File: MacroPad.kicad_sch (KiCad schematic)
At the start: 29 parts, among them SW1 RotaryEncoder_Switch, SW12 RotaryEncoder_Switch, SW2 RotaryEncoder_Switch, U1 Pico

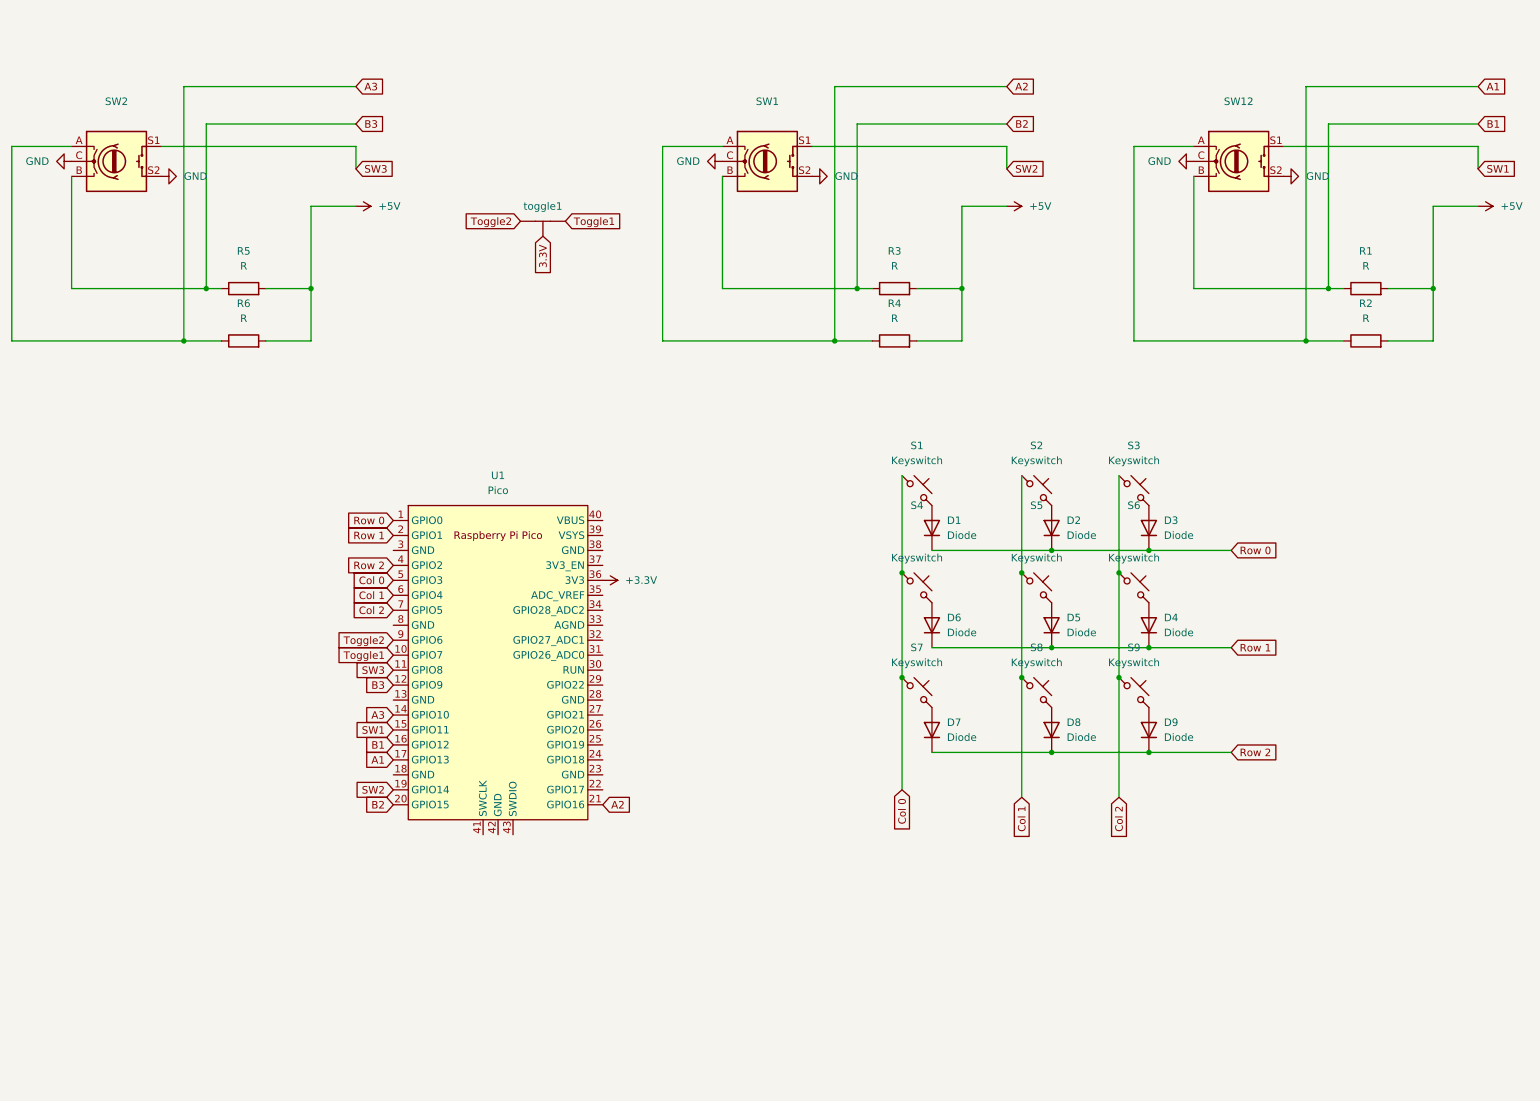
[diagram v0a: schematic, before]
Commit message: Redid the schematic should be finished
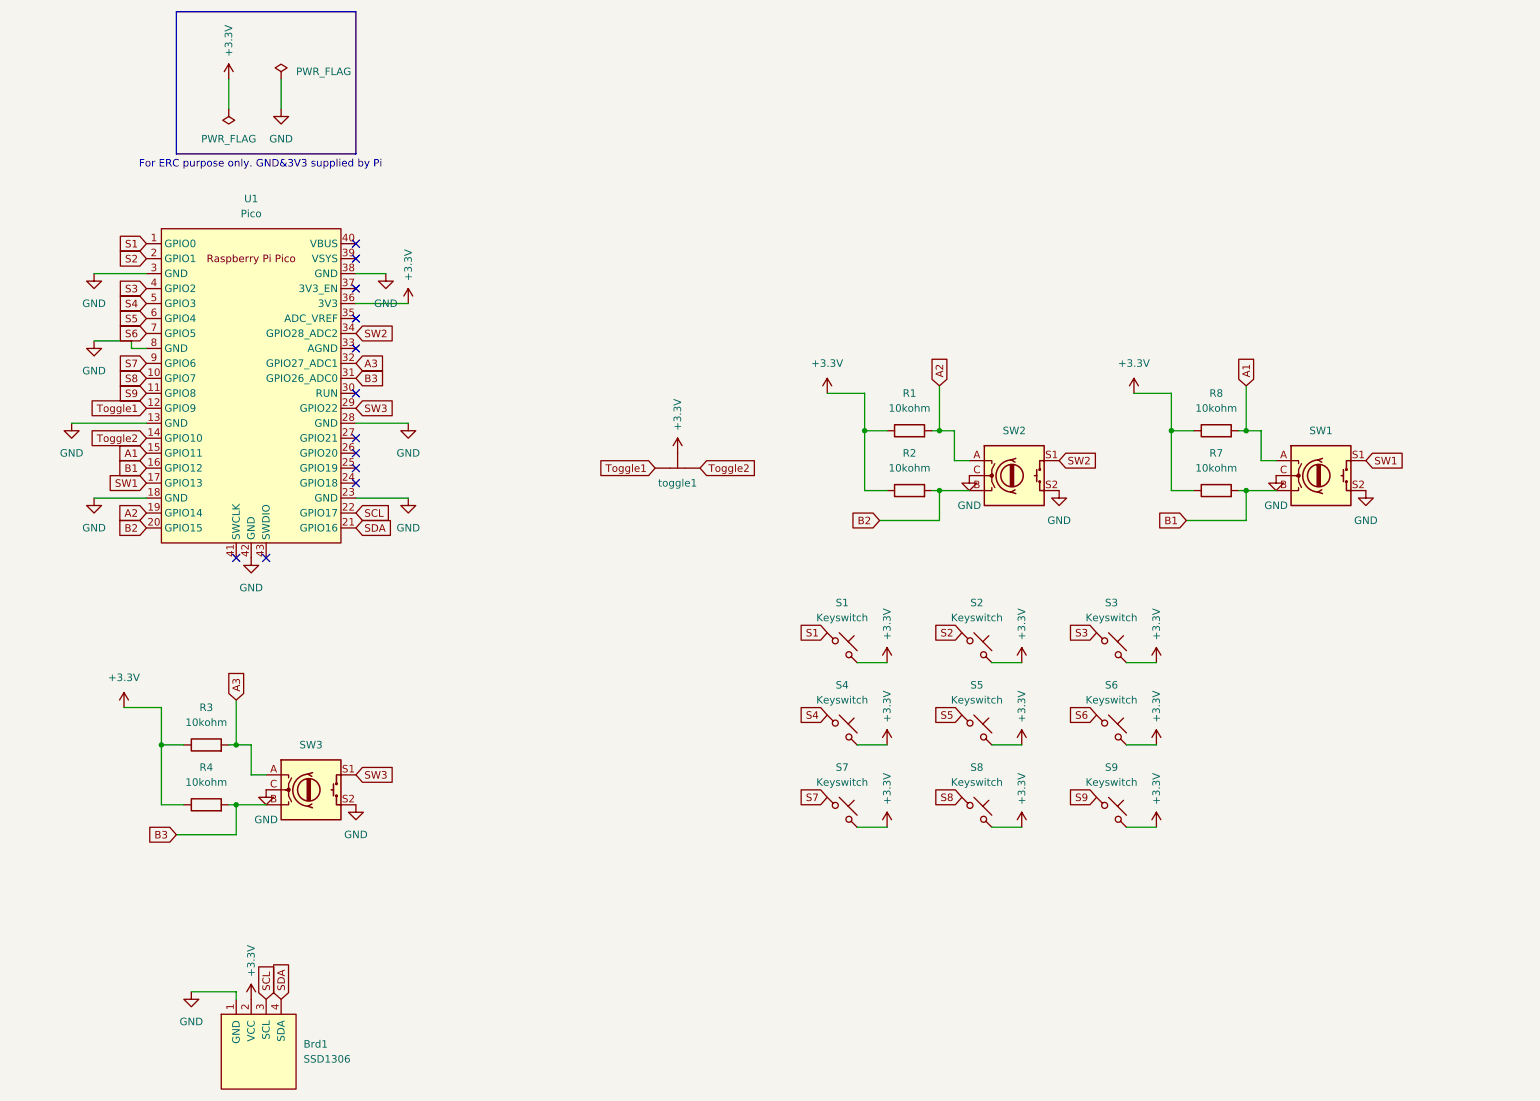
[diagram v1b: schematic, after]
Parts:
- removed D1, D2, D3, D4, D5, D6, D7, D8, D9: Diode, s_components:Diode_DO-35, symbol Scotto keedbs:Placeholder_Diode
- removed R5, R6: R, Resistor_THT:R_Axial_DIN0204_L3.6mm_D1.6mm_P7.62mm_Horizontal, symbol Device:R
- removed SW12: RotaryEncoder_Switch, Rotary_Encoder:RotaryEncoder_Alps_EC11E-Switch_Vertical_H20mm, symbol Device:RotaryEncoder_Switch
- added Brd1: SSD1306, dsada:128x64OLED, symbol dis:SSD1306
- added R7, R8: 10kohm, Resistor_THT:R_Axial_DIN0204_L3.6mm_D1.6mm_P7.62mm_Horizontal, symbol Device:R
- added SW3: RotaryEncoder_Switch, Rotary_Encoder:RotaryEncoder_Alps_EC11E-Switch_Vertical_H20mm, symbol Device:RotaryEncoder_Switch
- R1, R2, R3, R4: value R -> 10kohm
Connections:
- net 3.3V is gone; now on net Toggle2: toggle1.
- net +3.3V: now also R1.1, R2.1, R3.1, R4.1, S1.2, S2.2, S3.2, S4.2, S5.2, S6.2, S7.2, S8.2, S9.2, toggle1., Brd1.2 (VCC), R7.1, R8.1
- net A1: now also SW1.A, U1.15 (GPIO11), R8.2; no longer R2.1, U1.17 (GPIO13)
- net A2: now also R1.2, SW2.A, U1.19 (GPIO14); no longer R4.1, SW1.A, U1.21 (GPIO16)
- net A3: now also R3.2, U1.32 (GPIO27_ADC1), SW3.A; no longer SW2.A, U1.14 (GPIO10)
- net B1: now also SW1.B, R7.2; no longer R1.1
- net B2: now also R2.2, SW2.B; no longer R3.1, SW1.B
- net B3: now also R4.2, U1.31 (GPIO26_ADC0), SW3.B; no longer SW2.B, U1.12 (GPIO9)
- net GND: now also U1.13 (GND), U1.18 (GND), U1.23 (GND), U1.28 (GND), U1.3 (GND), U1.38 (GND), U1.42 (GND), U1.8 (GND), Brd1.1 (GND), SW3.C, SW3.S2
- net SW1: now also SW1.S1, U1.17 (GPIO13); no longer U1.15 (GPIO11)
- net SW2: now also SW2.S1, U1.34 (GPIO28_ADC2); no longer SW1.S1, U1.19 (GPIO14)
- net SW3: now also U1.29 (GPIO22), SW3.S1; no longer SW2.S1, U1.11 (GPIO8)
- net Toggle1: now also U1.12 (GPIO9); no longer U1.10 (GPIO7)
- net Toggle2: now also U1.14 (GPIO10); no longer U1.9 (GPIO6)
- net SCL: now reaches U1.22 (GPIO17)
- net SCL: now also Brd1.3 (SCL)
- removed net +5V: R1.2, R2.2, R3.2, R4.2
- net Col 0 renamed S4
- net S4: no longer S1.1, S7.1
- net Col 1 renamed S5
- net S5: no longer S2.1, S8.1
- net Col 2 renamed S6
- net S6: no longer S3.1, S9.1
- net Row 0 renamed S1
- net S1: now also S1.1
- net Row 1 renamed S2
- net S2: now also S2.1
- net Row 2 renamed S3
- net S3: now also S3.1
- new net S7: S7.1, U1.9 (GPIO6)
- new net S8: S8.1, U1.10 (GPIO7)
- new net S9: S9.1, U1.11 (GPIO8)
- new net SDA: Brd1.4 (SDA), U1.21 (GPIO16)
- no-connect marks 0 -> 12
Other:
- note added: "For ERC purpose only. GND&3V3 supplied by Pi"
- moved on the sheet: U1, toggle1

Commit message: Electric test work
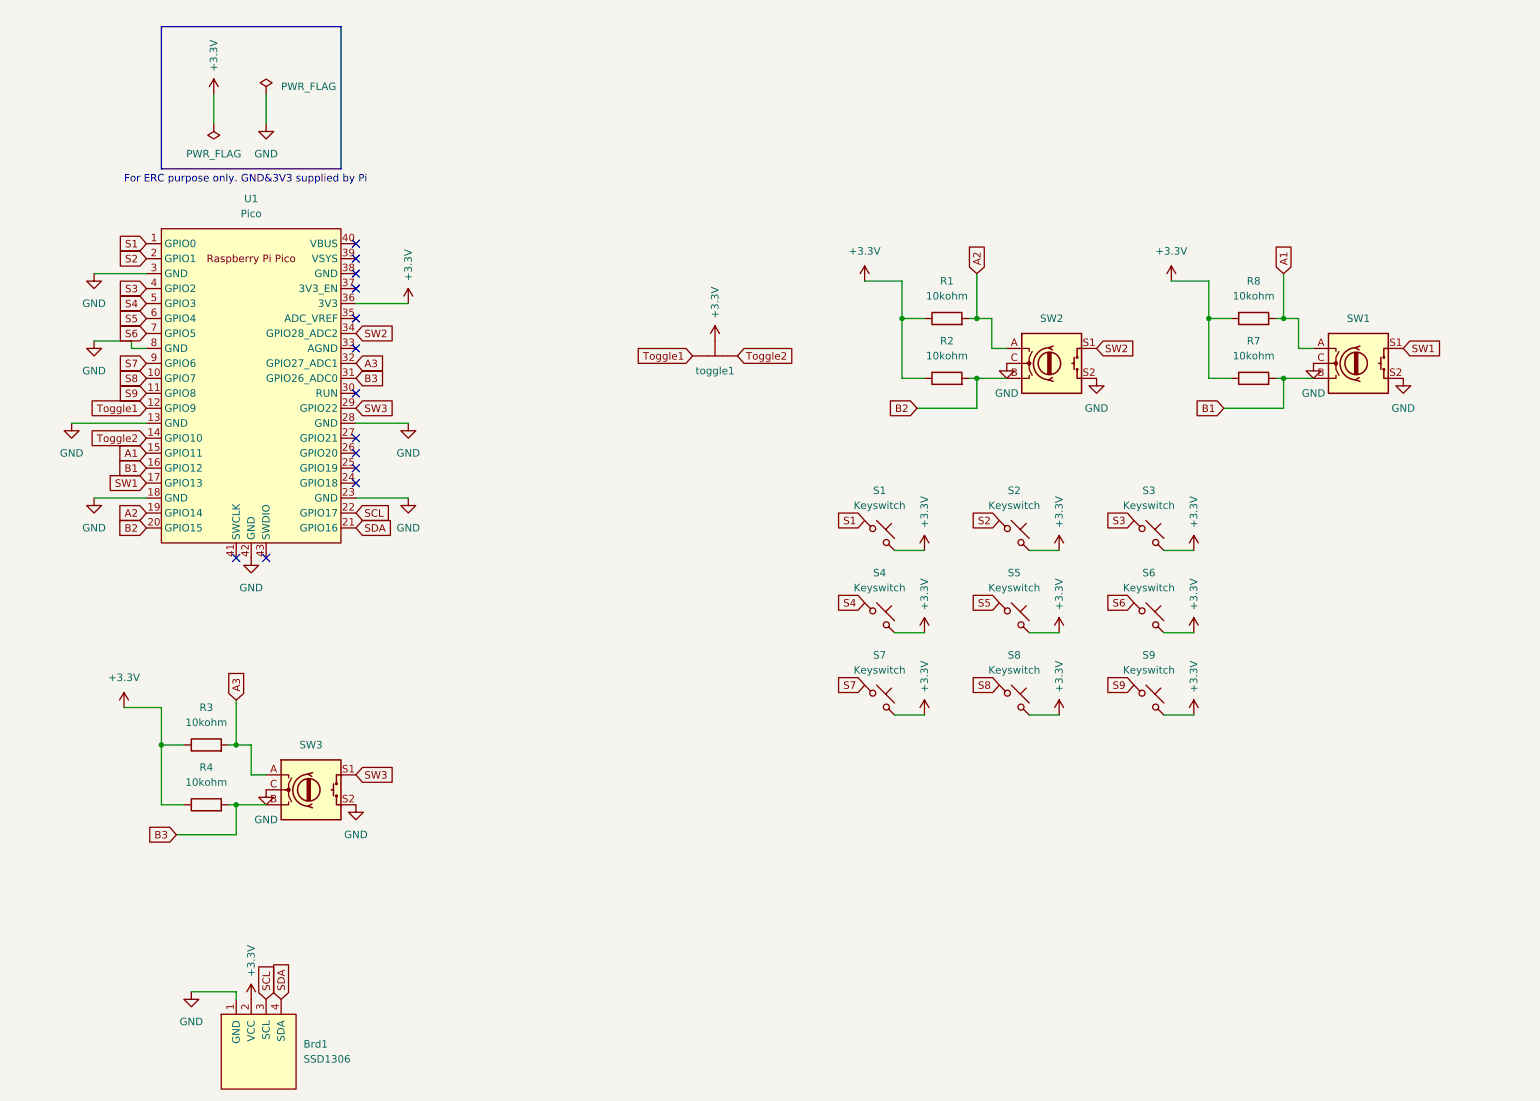
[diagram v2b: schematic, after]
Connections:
- net GND: no longer U1.38 (GND)
- no-connect marks 12 -> 13
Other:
- moved on the sheet: R1, R2, R7, R8, S1, S2, S3, S4, S5, S6, S7, S8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
